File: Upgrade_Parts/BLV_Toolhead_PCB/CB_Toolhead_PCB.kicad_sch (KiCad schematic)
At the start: 11 parts, among them J1 Micro-Fit, J2 JST-4, J3 JST-2, J4 JST-2, J5 JST-2, J6 JST-2, J7 Endstop, J8 JST-3, J9 JST-2

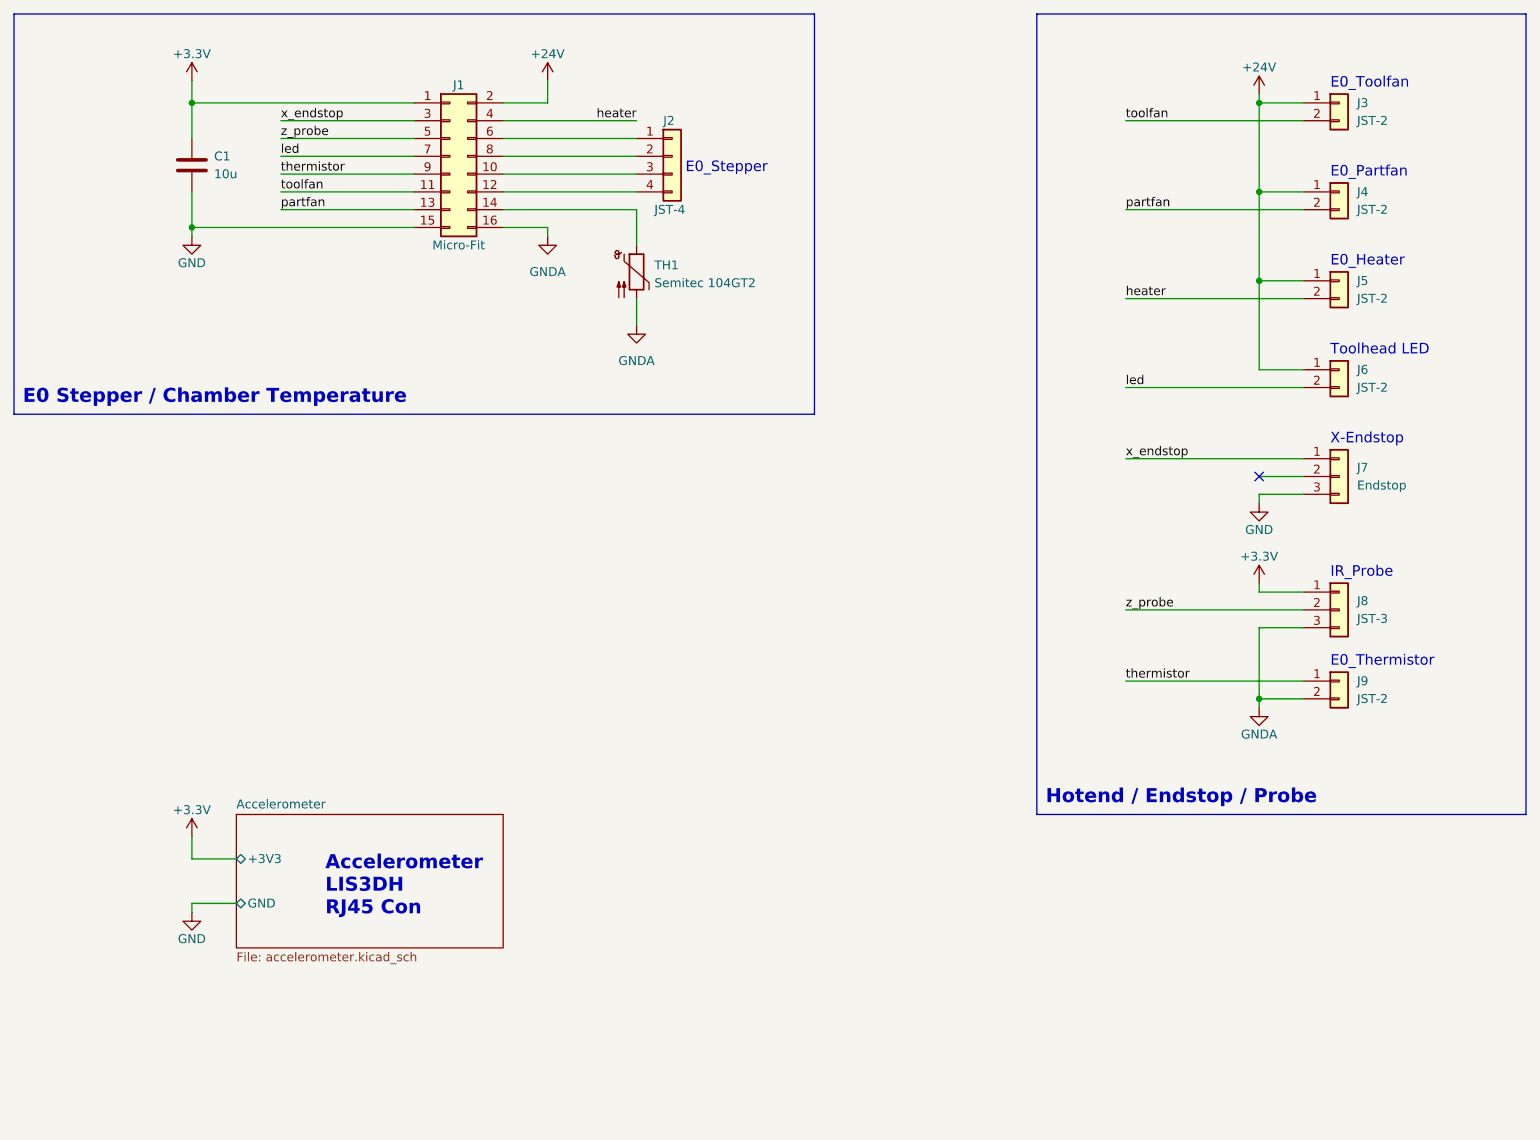
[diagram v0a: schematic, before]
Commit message: cleanup
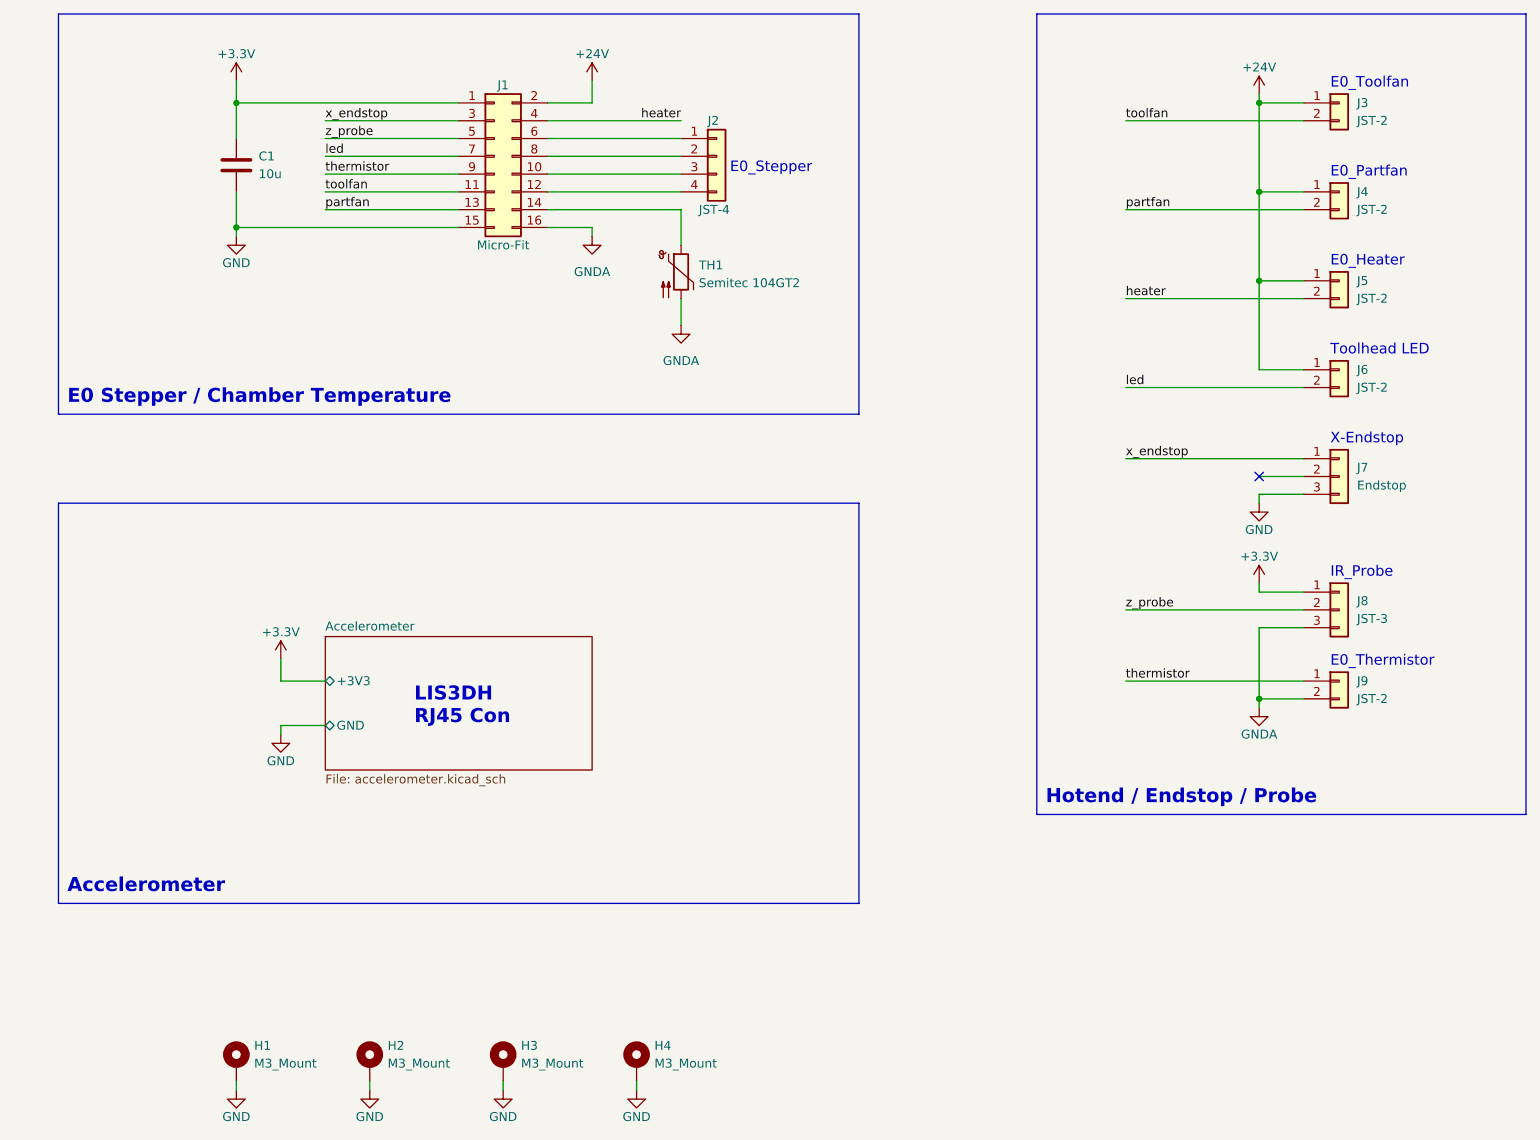
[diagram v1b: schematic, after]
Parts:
- added H1, H2, H3, H4: M3_Mount, symbol Mechanical:MountingHole_Pad
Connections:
- net GND: now also H1.1, H2.1, H3.1, H4.1
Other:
- note added: "Accelerometer"
- note added: "LIS3DH RJ45 Con"
- note removed: "Accelerometer LIS3DH RJ45 Con"
- moved on the sheet: C1, J1, J2, TH1
